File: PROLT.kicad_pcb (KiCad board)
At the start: 4 copper layers, 80 x 80 mm, 82 parts, among them IC1 BTS4175SGA, IC2 IFX9201SGAUMA1, IC3 IFX9201SGAUMA1, J1 64334-0100, J2 USB, M1 Module:mega-mcu100/0.3, M2 Module-vr-max9924-0.1, M3 Module-power_12and5V-0.2, U1 JDY-33, U2 VNLD5160TR-E, U3 VNLD5160TR-E, U4 VNLD5160TR-E

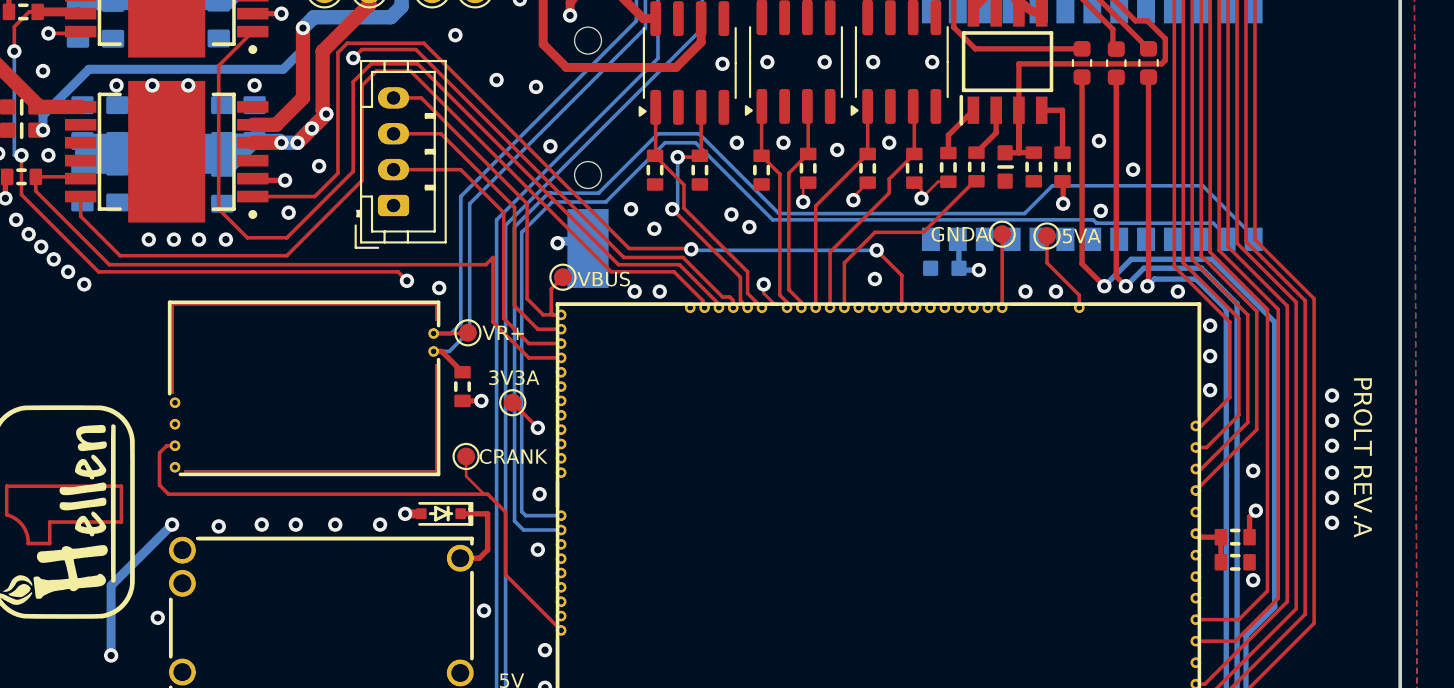
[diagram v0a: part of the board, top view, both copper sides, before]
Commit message: Rev B
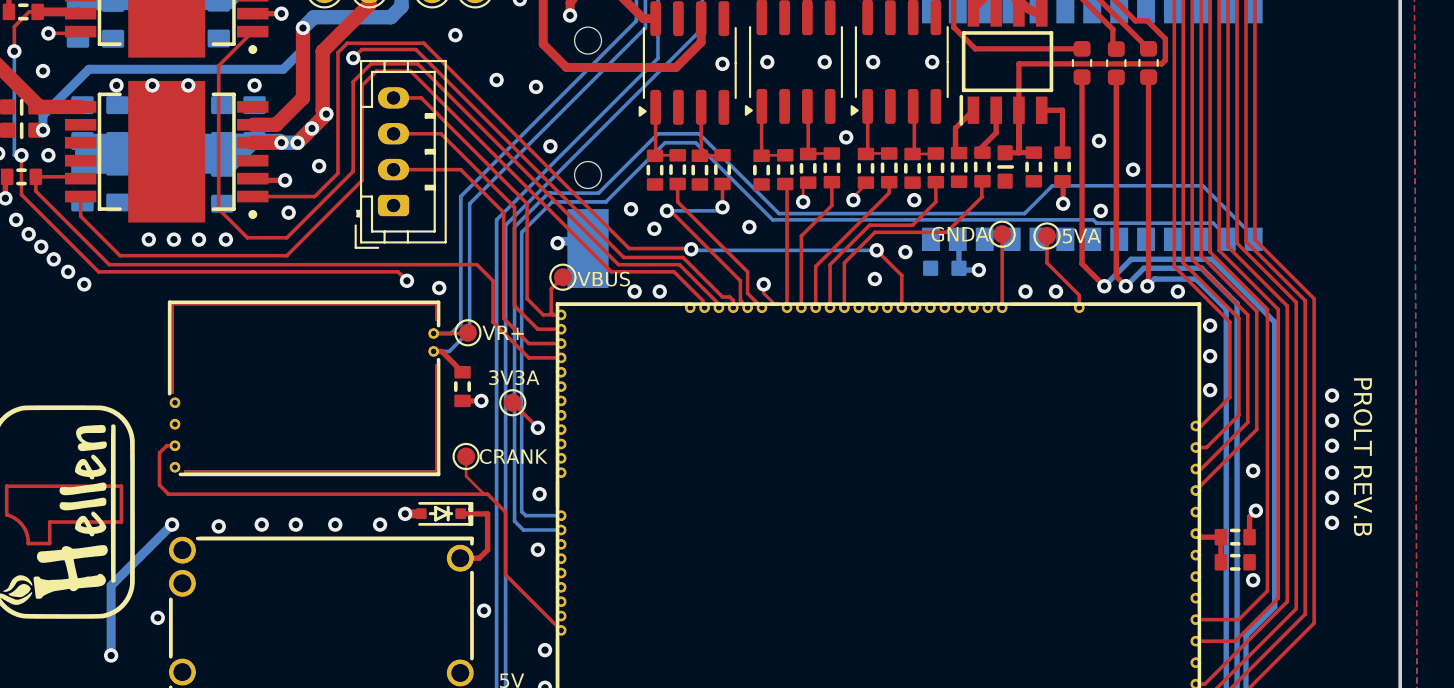
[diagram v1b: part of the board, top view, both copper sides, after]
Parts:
- added R17: 4.7k, Hellen:R0603, F.Cu at (155.0, 91.1)
- added R18: 4.7k, Hellen:R0603, F.Cu at (152.4, 91.2)
- added R19: 4.7k, Hellen:R0603, F.Cu at (158.2, 91.1)
- added R20: 4.7k, Hellen:R0603, F.Cu at (160.8, 91.1)
- added R21: 4.7k, Hellen:R0603, F.Cu at (146.4, 91.2)
- added R22: 4.7k, Hellen:R0603, F.Cu at (148.9, 91.2)
- C28: value 100nF -> 100n
- R5: value 10k -> 150
- R6: value 10k -> 0R
- R7: value 10k -> 15k
- moved R5 0.60 mm to (162.1, 91.1)
- moved R6 0.34 mm to (163.4, 91.0)
- moved R3 0.10 mm to (156.9, 91.1)
- moved R4 0.10 mm to (159.5, 91.1)
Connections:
- R1 pad 2: /INJ1_IN -> Net-(U2-IN1)
- R10 pad 2: /LS2 -> Net-(U4-IN2)
- R2 pad 2: /INJ2_IN -> Net-(U2-IN2)
- R3 pad 2: /INJ3_IN -> Net-(U3-IN1)
- R4 pad 2: /INJ4_IN -> Net-(U3-IN2)
- R9 pad 2: /LS1 -> Net-(U4-IN1)
- U2 pad 1: /INJ1_IN -> Net-(U2-IN1)
- U2 pad 3: /INJ2_IN -> Net-(U2-IN2)
- U3 pad 1: /INJ3_IN -> Net-(U3-IN1)
- U3 pad 3: /INJ4_IN -> Net-(U3-IN2)
- U4 pad 1: /LS1 -> Net-(U4-IN1)
- U4 pad 3: /LS2 -> Net-(U4-IN2)
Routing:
- net /INJ1_IN: track 11.8 -> 6.94 mm
- net /LS1: track 13.7 -> 8.85 mm
- net /INJ2_IN: track 12.0 -> 7.70 mm
- net Net-(U4-IN2): track 0.00 -> 4.15 mm
- net Net-(U2-IN1): track 0.00 -> 4.10 mm
- net Net-(U2-IN2): track 0.00 -> 4.03 mm
- net Net-(U3-IN2): track 0.00 -> 4.03 mm
- net Net-(U4-IN1): track 0.00 -> 4.02 mm
- net Net-(U3-IN1): track 0.00 -> 3.97 mm
- net /INJ3_IN: track 12.4 -> 8.70 mm
- net GND: track 10.8 -> 7.89 mm, vias 165 -> 162
- net /LS2: track 14.5 -> 11.9 mm
- net /INJ4_IN: track 13.2 -> 10.8 mm
- net /DC2_DIS: track 38.9 -> 37.8 mm
- net /HS: track 11.7 -> 12.6 mm
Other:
- board text added: "PROLT REV.B"
- board text removed: "PROLT REV.A"
